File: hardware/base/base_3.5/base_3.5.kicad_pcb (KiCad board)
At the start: 2 copper layers, 82.4 x 17 mm, 5 parts, among them J1 Conn 1, J2 Conn 2, J3 Conn_01x03, J4 Conn_01x03

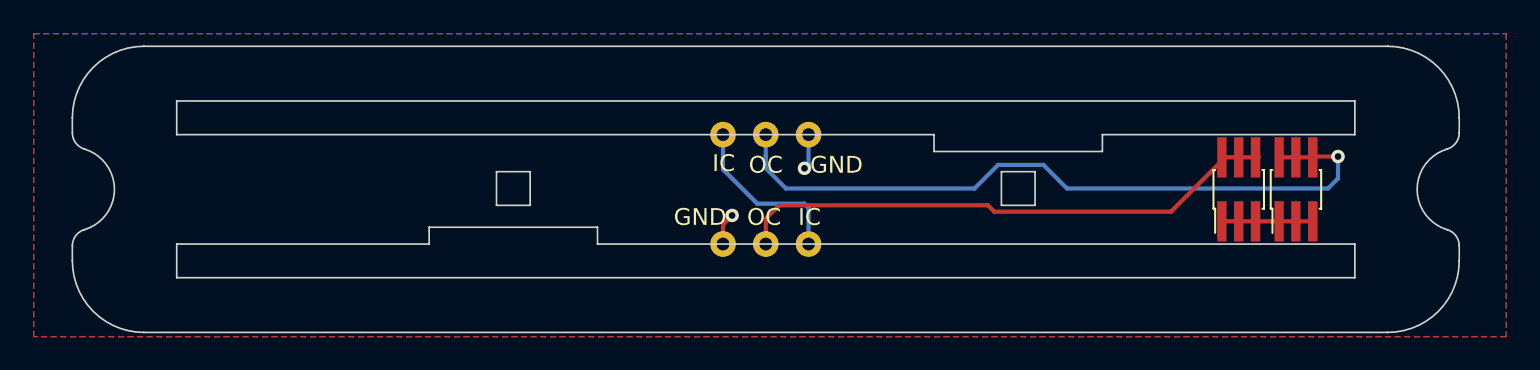
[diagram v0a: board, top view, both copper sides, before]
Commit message: 3.0 and 3.5 base updated
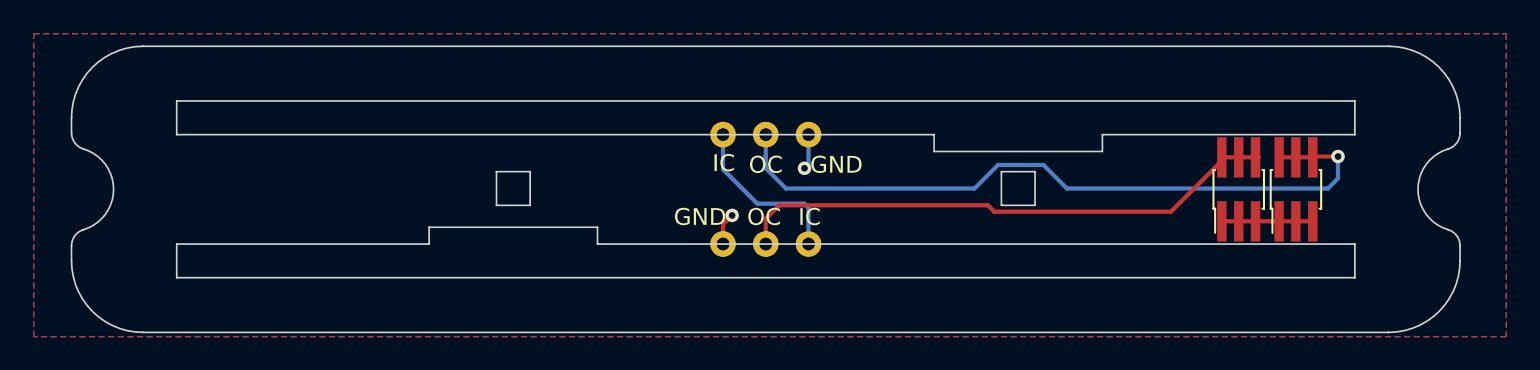
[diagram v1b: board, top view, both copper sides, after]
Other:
- board size 82.4 x 17 mm -> 82.5 x 17 mm
